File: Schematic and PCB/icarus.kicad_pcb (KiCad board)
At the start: 2 copper layers, 35 x 50 mm, 56 parts, among them J1 Conn_01x02_Socket, J2 USB_C_Receptacle_USB2.0_16P, J3 Conn_01x02_Socket, J4 Conn_01x02_Socket, J5 Conn_01x02_Socket, J6 Conn_01x02_Socket, J8 Conn_01x02_Pin, Q1 AO3400A, Q2 AO3400A, Q3 AO3400A, Q4 AO3400A, SW1 SW_Push(BOOt), U2 BMI088, U3 AMS1117-3.3, U4 ESP32-S3-WROOM-1

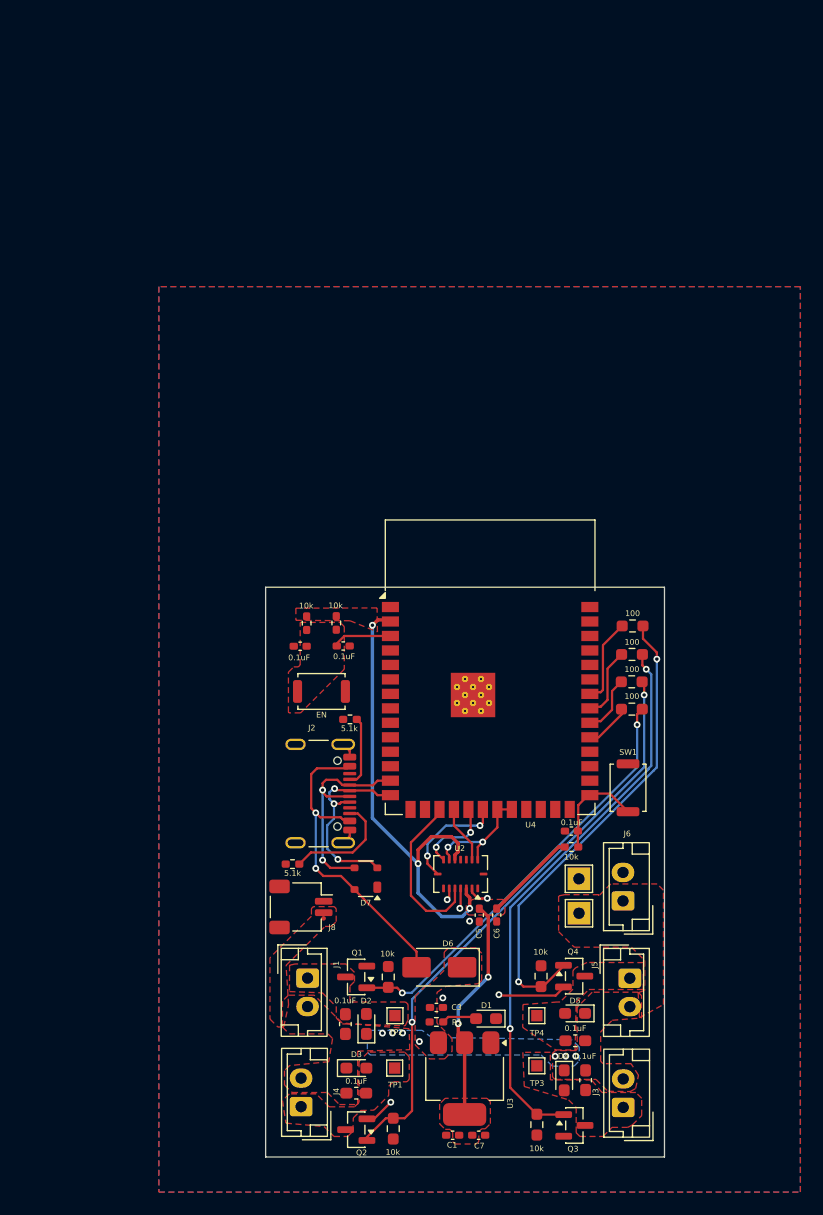
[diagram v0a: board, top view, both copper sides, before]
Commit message: FINAL PCB
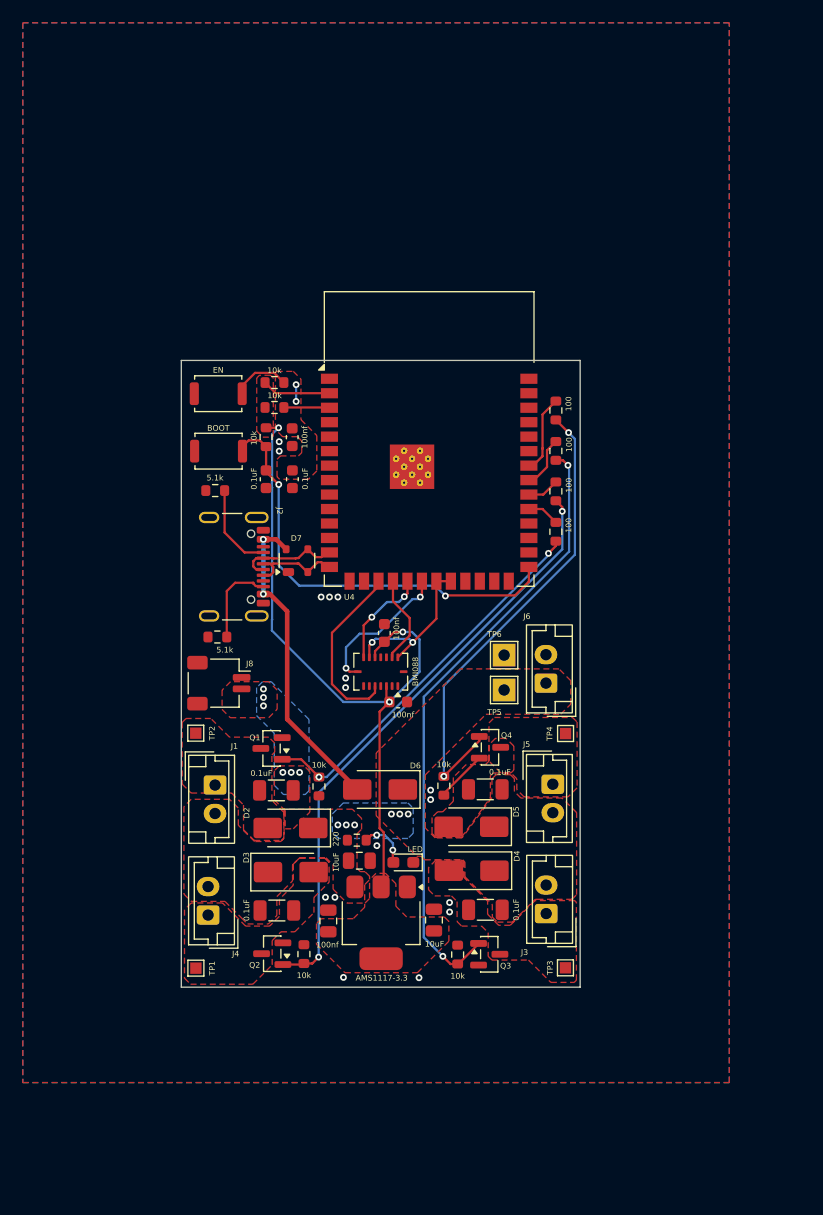
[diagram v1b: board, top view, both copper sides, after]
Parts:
- removed 0.1uF (x2): 0.1uF, Capacitor_SMD:C_0402_1005Metric_Pad0.74x0.62mm_HandSolder
- removed 0.1uF (x4): 0.1uF, Capacitor_SMD:C_0603_1608Metric_Pad1.08x0.95mm_HandSolder
- removed 0.1uF: 100nf, Capacitor_SMD:C_0402_1005Metric_Pad0.74x0.62mm_HandSolder
- removed 100: R6, Resistor_SMD:R_0603_1608Metric_Pad0.98x0.95mm_HandSolder
- removed 100: R4, Resistor_SMD:R_0603_1608Metric_Pad0.98x0.95mm_HandSolder
- removed 100: R7, Resistor_SMD:R_0603_1608Metric_Pad0.98x0.95mm_HandSolder
- removed 100: R5, Resistor_SMD:R_0603_1608Metric_Pad0.98x0.95mm_HandSolder
- removed 10k (x4): 10k, Resistor_SMD:R_0603_1608Metric_Pad0.98x0.95mm_HandSolder
- removed 10k: R3, Resistor_SMD:R_0402_1005Metric_Pad0.72x0.64mm_HandSolder
- removed 10k: 10k, Resistor_SMD:R_0402_1005Metric_Pad0.72x0.64mm_HandSolder
- removed 10k: R12, Resistor_SMD:R_0402_1005Metric_Pad0.72x0.64mm_HandSolder
- removed 5.1k (x2): 5.1k, Resistor_SMD:R_0402_1005Metric_Pad0.72x0.64mm_HandSolder
- removed SW1: SW_Push(BOOt), Button_Switch_SMD:SW_Push_SPST_NO_Alps_SKRK
- added BOOT: SW_Push(BOOt), Button_Switch_SMD:SW_Push_SPST_NO_Alps_SKRK, F.Cu at (125.3, 72.5)
- added C10: 0.1uF, Capacitor_SMD:C_1206_3216Metric, F.Cu at (130.3, 102.2)
- added C11: 0.1uF, Capacitor_SMD:C_1206_3216Metric, F.Cu at (148.7, 102.1)
- added C12: 0.1uF, Capacitor_SMD:C_1206_3216Metric, F.Cu at (148.7, 112.7)
- added C13: 0.1uF, Capacitor_SMD:C_1206_3216Metric, F.Cu at (130.4, 112.8)
- added C2: 0.1uF, Capacitor_SMD:C_0603_1608Metric, F.Cu at (129.4, 74.9)
- added C4: 0.1uF, Capacitor_SMD:C_0603_1608Metric, F.Cu at (131.8, 74.9)
- added C9: 100nf, Capacitor_SMD:C_0603_1608Metric, F.Cu at (131.7, 71.2)
- added R10: 10k, Resistor_SMD:R_0603_1608Metric, F.Cu at (146.2, 116.6)
- added R11: 10k, Resistor_SMD:R_0603_1608Metric, F.Cu at (145.0, 101.8)
- added R12: 10k, Resistor_SMD:R_0603_1608Metric, F.Cu at (130.2, 66.4)
- added R13: 5.1k, Resistor_SMD:R_0603_1608Metric, F.Cu at (125.0, 75.9)
- added R14: 5.1k, Resistor_SMD:R_0603_1608Metric, F.Cu at (125.2, 88.8)
- added R2: 10k, Resistor_SMD:R_0603_1608Metric, F.Cu at (129.4, 71.2)
- added R3: 10k, Resistor_SMD:R_0603_1608Metric, F.Cu at (130.2, 68.6)
- added R4: 100, Resistor_SMD:R_0603_1608Metric, F.Cu at (154.9, 79.5)
- added R5: 100, Resistor_SMD:R_0603_1608Metric, F.Cu at (154.9, 76.0)
- added R6: 100, Resistor_SMD:R_0603_1608Metric, F.Cu at (154.9, 72.4)
- added R7: 100, Resistor_SMD:R_0603_1608Metric, F.Cu at (154.9, 68.9)
- added R8: 10k, Resistor_SMD:R_0603_1608Metric, F.Cu at (134.1, 101.9)
- added R9: 10k, Resistor_SMD:R_0603_1608Metric, F.Cu at (132.8, 116.6)
- C1, C3, C7: footprint Capacitor_SMD:C_0402_1005Metric_Pad0.74x0.62mm_HandSolder -> Capacitor_SMD:C_0805_2012Metric
- C5, C6: footprint Capacitor_SMD:C_0402_1005Metric_Pad0.74x0.62mm_HandSolder -> Capacitor_SMD:C_0603_1608Metric
- D2, D3, D4, D5: value 1N5819 -> SS24; footprint Diode_SMD:D_0603_1608Metric_Pad1.05x0.95mm_HandSolder -> Diode_SMD:D_SMA
- R1: value 220ohm -> 220; footprint Resistor_SMD:R_0402_1005Metric_Pad0.72x0.64mm_HandSolder -> Resistor_SMD:R_0603_1608Metric
- moved TP2 30.3 mm to (123.3, 97.2), turned to 0 degrees
- moved D7 28.6 mm to (132.2, 82.1), turned to 90 degrees
- moved EN 27.7 mm to (125.2, 67.4), turned to 0 degrees
- moved C6 26.6 mm to (139.8, 88.4), turned to 90 degrees
- moved TP4 24.9 mm to (155.7, 97.2), turned to 0 degrees
- moved C7 23.0 mm to (134.9, 113.7), turned to 90 degrees
- moved Q4 21.4 mm to (149.1, 98.5)
- moved Q1 21.4 mm to (129.9, 98.5)
- moved J2 21.3 mm to (125.5, 82.6)
- moved J8 20.9 mm to (125.3, 92.8)
- moved U4 20.7 mm to (143.8, 71.4)
- moved TP6 20.7 mm to (150.3, 90.4), turned to 180 degrees
- moved TP5 20.7 mm to (150.3, 93.4), turned to 180 degrees
- moved J6 20.3 mm to (154.0, 92.8)
- moved D4 20.1 mm to (147.5, 109.3), turned to 180 degrees
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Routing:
- net /BOOT: track 9.05 -> 38.1 mm, vias 0 -> 2
- net GND: track 16.5 -> 4.40 mm, vias 7 -> 16
- net /USB_D-: track 18.7 -> 8.69 mm, vias 2 -> 0
- net /USB_D+: track 17.2 -> 8.76 mm, vias 3 -> 0
- net /M3: track 48.9 -> 54.5 mm
- net /EN: track 5.04 -> 9.94 mm, vias 0 -> 2
- net /M1: track 37.6 -> 33.6 mm
- net /SD01: track 10.8 -> 14.6 mm
- net /SCK: track 9.95 -> 12.8 mm
- net /CSB1: track 5.21 -> 7.92 mm
- net Net-(U4-IO39): track 5.10 -> 2.83 mm
- net Net-(J2-CC2): track 9.99 -> 7.72 mm
- net Net-(U4-IO40): track 6.24 -> 4.18 mm
- net /SDI: track 6.99 -> 8.89 mm
- net Net-(J2-CC1): track 6.18 -> 7.80 mm
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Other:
- board size 35 x 50 mm -> 35 x 55 mm
